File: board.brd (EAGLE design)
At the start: 52 x 51.7 mm, 14 parts, among them J1 5.5x2.1mm Barrel, T1 TIP122

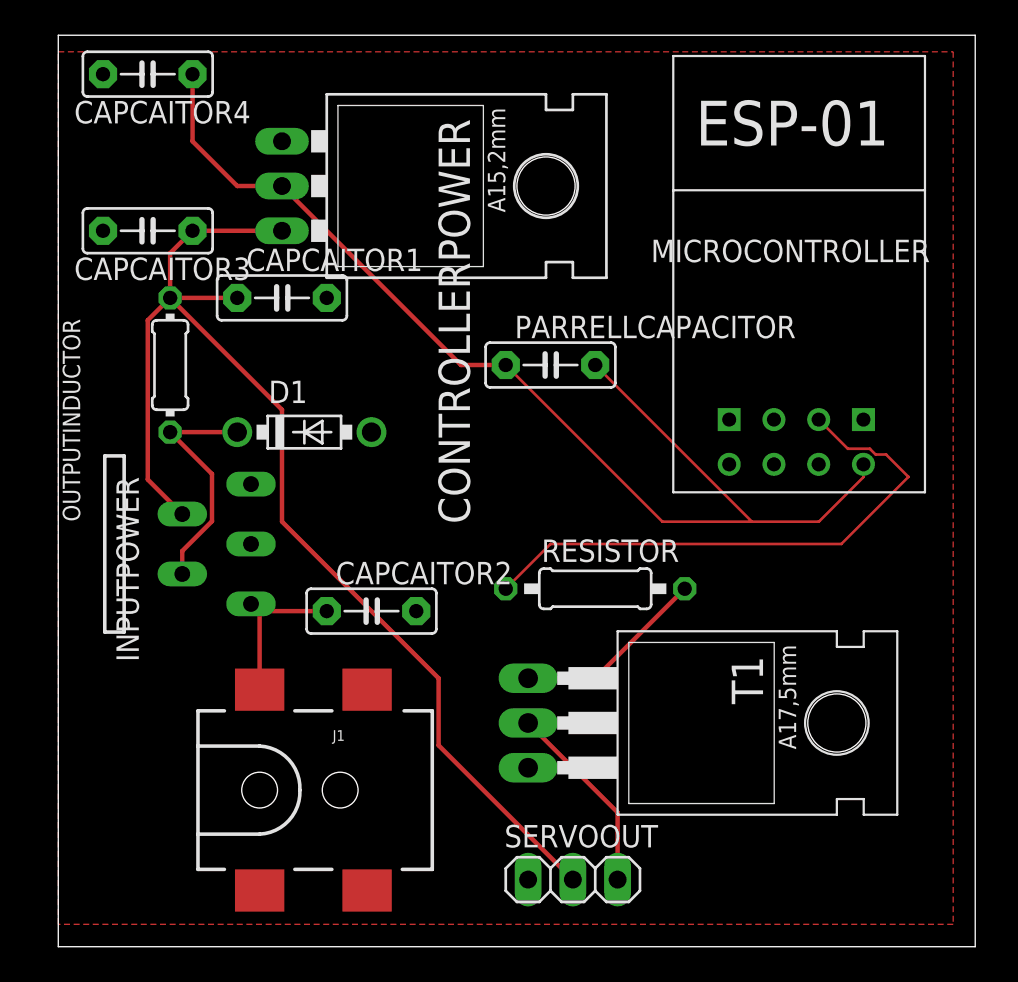
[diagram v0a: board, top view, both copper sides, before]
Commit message: Updated PCB and Gerber Files
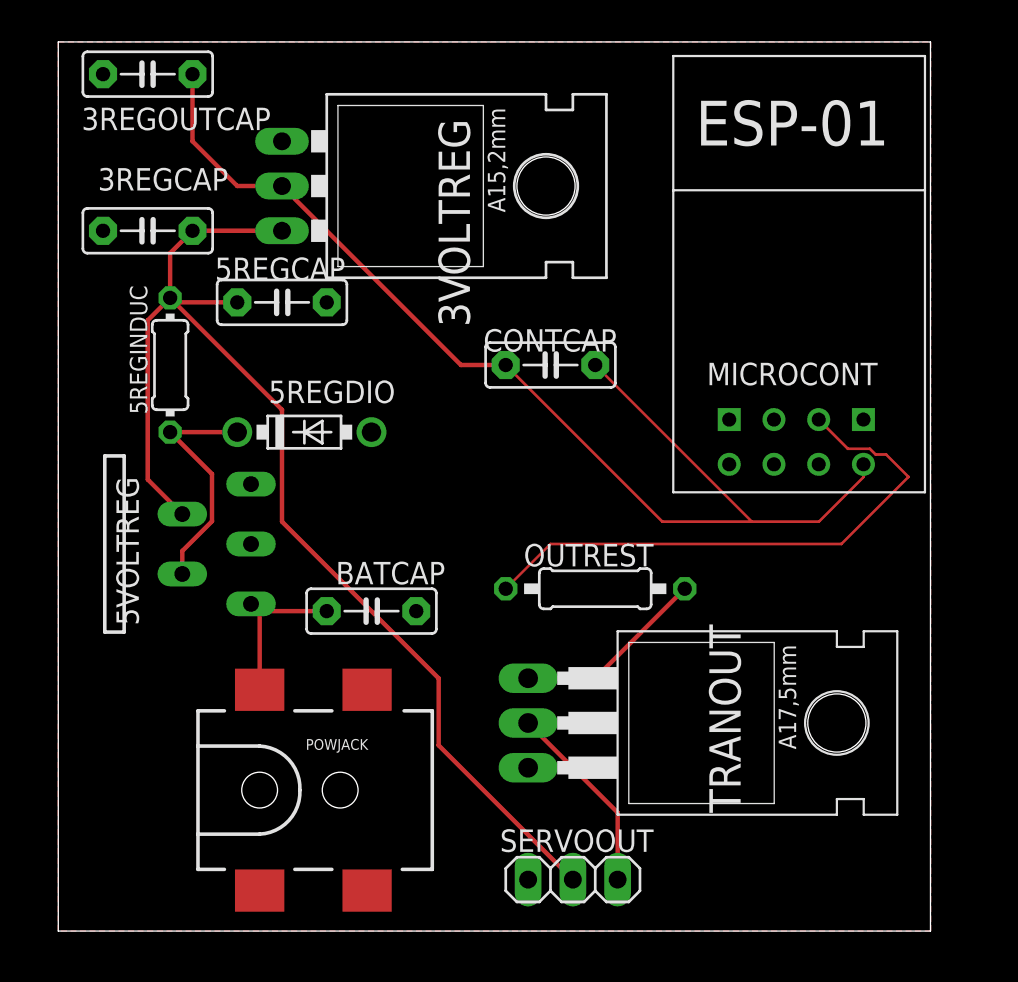
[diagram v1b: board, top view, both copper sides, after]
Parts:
- removed CAPCAITOR1: 1000uf, capacitor-wima:C5B2.5
- added 5REGCAP: 1000uf, capacitor-wima:C5B2.5
- renumbered CAPCAITOR2 to BATCAP, CAPCAITOR3 to 3REGCAP, CAPCAITOR4 to 3REGOUTCAP, CONTROLLERPOWER to 3VOLTREG, D1 to 5REGDIO, INPUTPOWER to 5VOLTREG, J1 to POWJACK, MICROCONTROLLER to MICROCONT, OUTPUTINDUCTOR to 5REGINDUC, PARRELLCAPACITOR to CONTCAP, RESISTOR to OUTREST, T1 to TRANOUT
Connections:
- net GND: now also 5REGCAP.2; no longer CAPCAITOR1.2
- net N$5: now also 5REGCAP.1; no longer CAPCAITOR1.1
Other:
- board size 52 x 51.7 mm -> 49.5 x 50.5 mm
